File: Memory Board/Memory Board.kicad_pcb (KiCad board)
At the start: 4 copper layers, 50.8 x 50.8 mm, 40 parts, among them IC1 W25Q01JVZEIQ, IC2 MCP2557FDT-H_MNY, J1 USB4056-03-A_REVA2, J2 Conn_01x04_Socket, J3 Conn_01x04_Socket, J4 Conn_01x04_Socket, SW1 SW_SPST, U1 STM32G473CBTx, U2 LD1117S33TR_SOT223, U3 LD1117S50TR_SOT223, X1 ECS-2520MV-xxx-xx

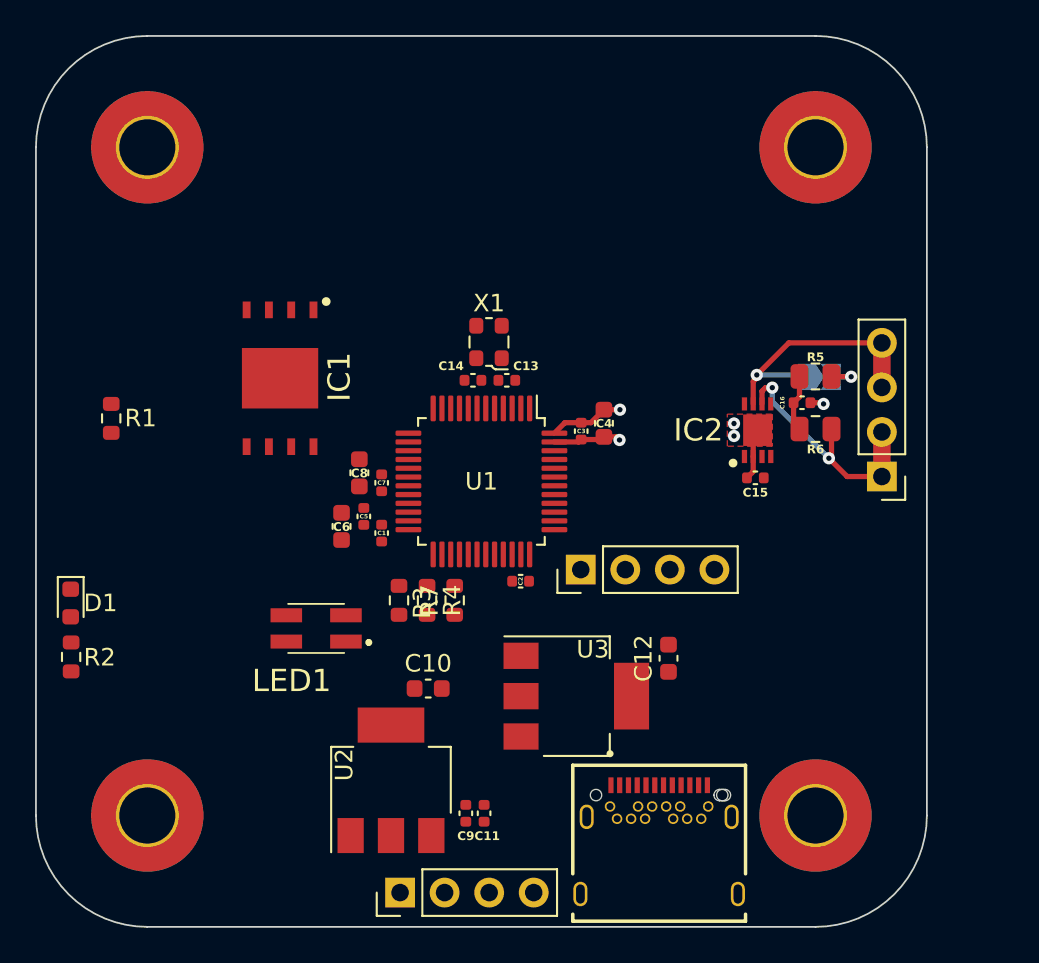
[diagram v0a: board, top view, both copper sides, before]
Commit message: Layout work
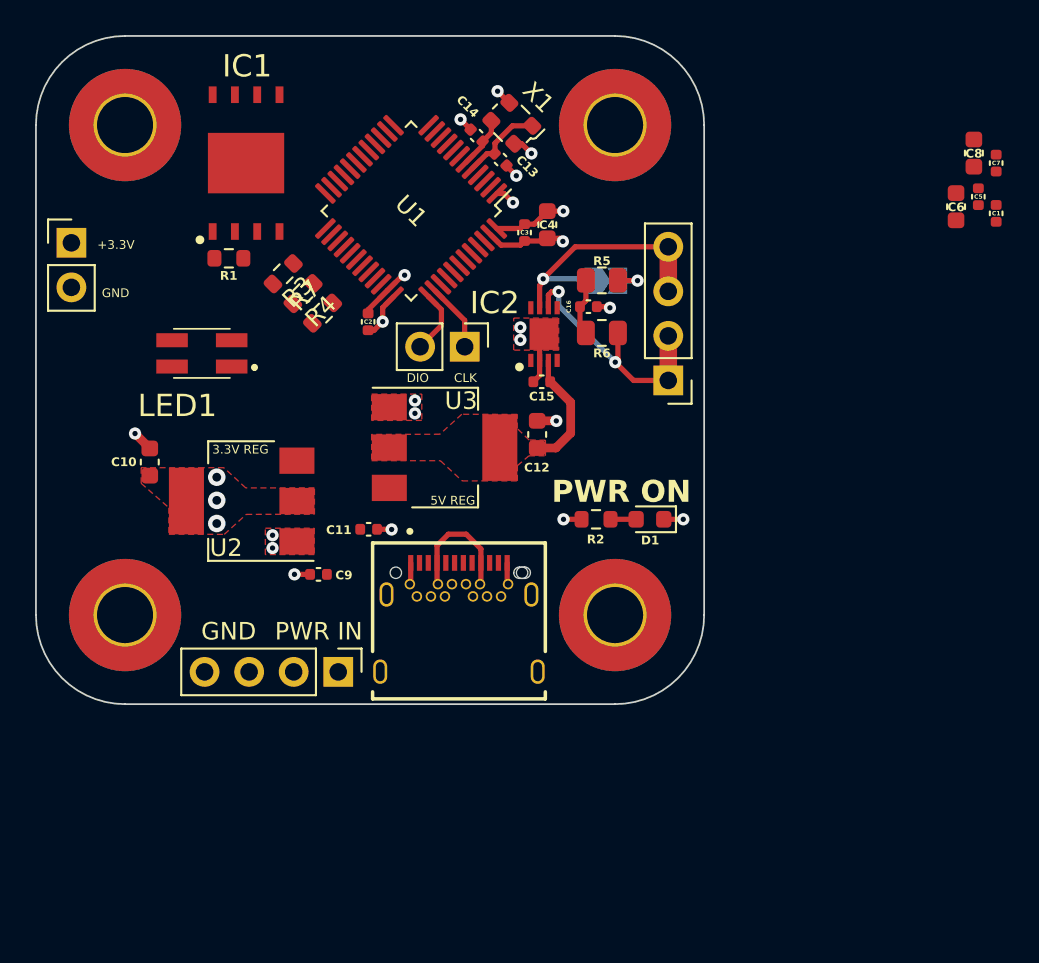
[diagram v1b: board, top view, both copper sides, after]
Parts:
- added J5: Conn_01x02_Socket, Connector_PinHeader_2.54mm:PinHeader_1x02_P2.54mm_Vertical, F.Cu at (27.4, 37.2)
- J4: value Conn_01x04_Socket -> Conn_01x02_Socket; footprint Connector_PinHeader_2.54mm:PinHeader_1x04_P2.54mm_Vertical -> Connector_PinHeader_2.54mm:PinHeader_1x02_P2.54mm_Vertical
- moved C1 39.5 mm to (80.2, 35.5)
- moved C6 39.5 mm to (77.9, 35.1)
- moved C7 39.5 mm to (80.2, 32.6)
- moved C5 39.5 mm to (79.1, 34.6)
- moved C8 39.5 mm to (78.9, 32.1)
- moved D1 33.4 mm to (60.4, 53.0), turned to 180 degrees
- moved R2 30.9 mm to (57.3, 53.0), turned to 0 degrees
- moved C10 20.5 mm to (31.9, 49.7), turned to 90 degrees
- moved R3 19.8 mm to (39.5, 39.0), turned to -135 degrees
- moved R4 18.9 mm to (40.6, 40.1), turned to -135 degrees
- moved U2 18.1 mm to (37.1, 51.9), turned to 180 degrees
- moved R7 18.0 mm to (41.7, 41.2), turned to 45 degrees
- moved C11 17.5 mm to (44.4, 53.5), turned to 0 degrees
- moved C2 17.2 mm to (44.3, 41.7), turned to 90 degrees
- moved J1 17.1 mm to (49.5, 61.6)
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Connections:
- J4 pad 1: SYS_SWDIO -> SYS_SWCLK
- J4 pad 2: GND -> SYS_SWDIO
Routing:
- net GND: track 7.65 -> 22.8 mm, vias 4 -> 18
- net PWR IN: track 0.00 -> 7.37 mm
- net +5V: track 0.00 -> 6.94 mm
- net +3.3V: track 4.29 -> 9.08 mm, vias 1 -> 7
- net RCC_OCC_IN: track 0.00 -> 4.78 mm
- net SYS_SWCLK: track 0.00 -> 3.91 mm
- net SYS_SWDIO: track 0.00 -> 3.66 mm
- net RCC_OCC_OUT: track 0.00 -> 2.98 mm
- net Net-(D1-A): track 0.00 -> 1.46 mm
- added copper zone on F.Cu, net +3.3V
- added copper zone on F.Cu, net +5V
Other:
- board size 50.8 x 50.8 mm -> 38.1 x 38.1 mm
- board text added: "+3.3V"
- board text added: "3.3V REG"
- board text added: "5V REG"
- board text added: "CLK"
- board text added: "DIO"
- board text added: "GND"
- board text added: "PWR IN"
- board text added: "PWR ON"
